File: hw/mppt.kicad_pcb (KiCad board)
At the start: 2 copper layers, 7 parts, among them J1 Conn_01x02, J2 Conn_01x02, Q1 Q_NMOS_DGS, Q2 Q_NMOS_DGS

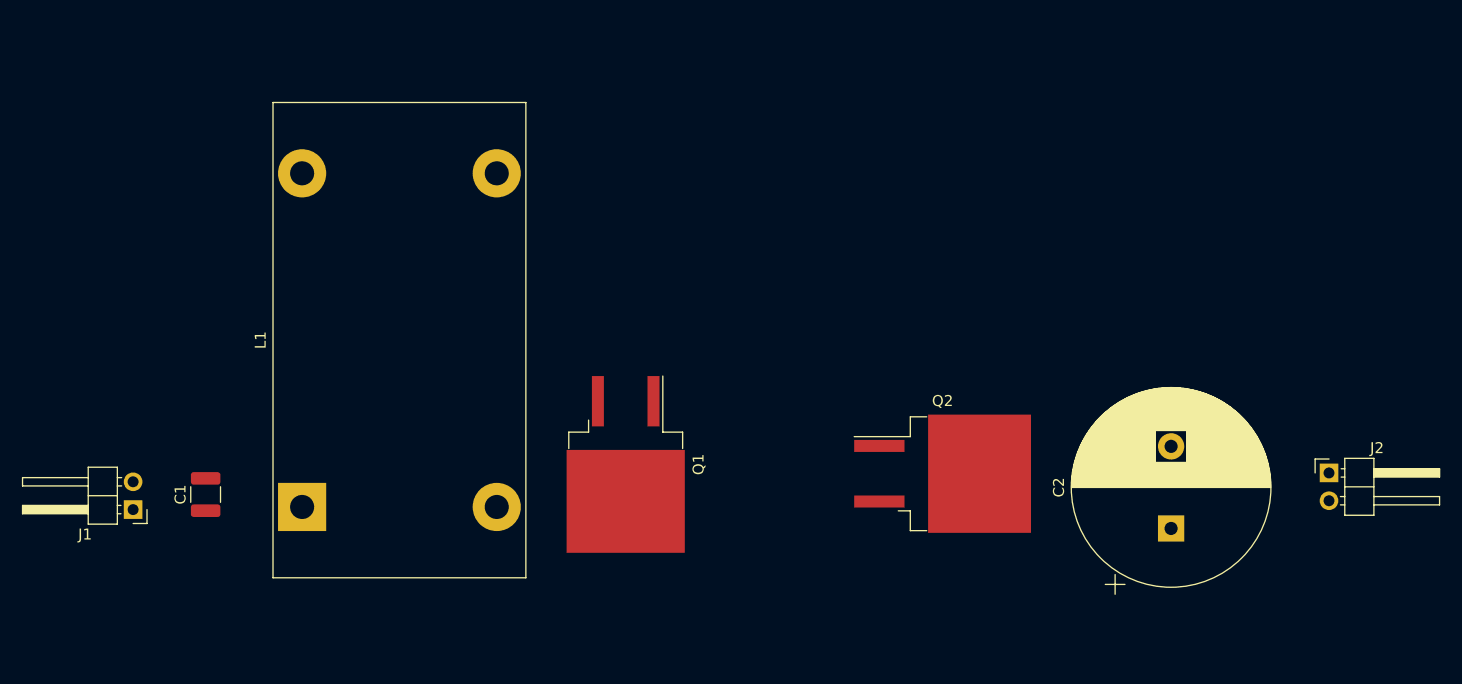
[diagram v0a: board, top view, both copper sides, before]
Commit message: working on documentation, design methmethodology, sizing, layout
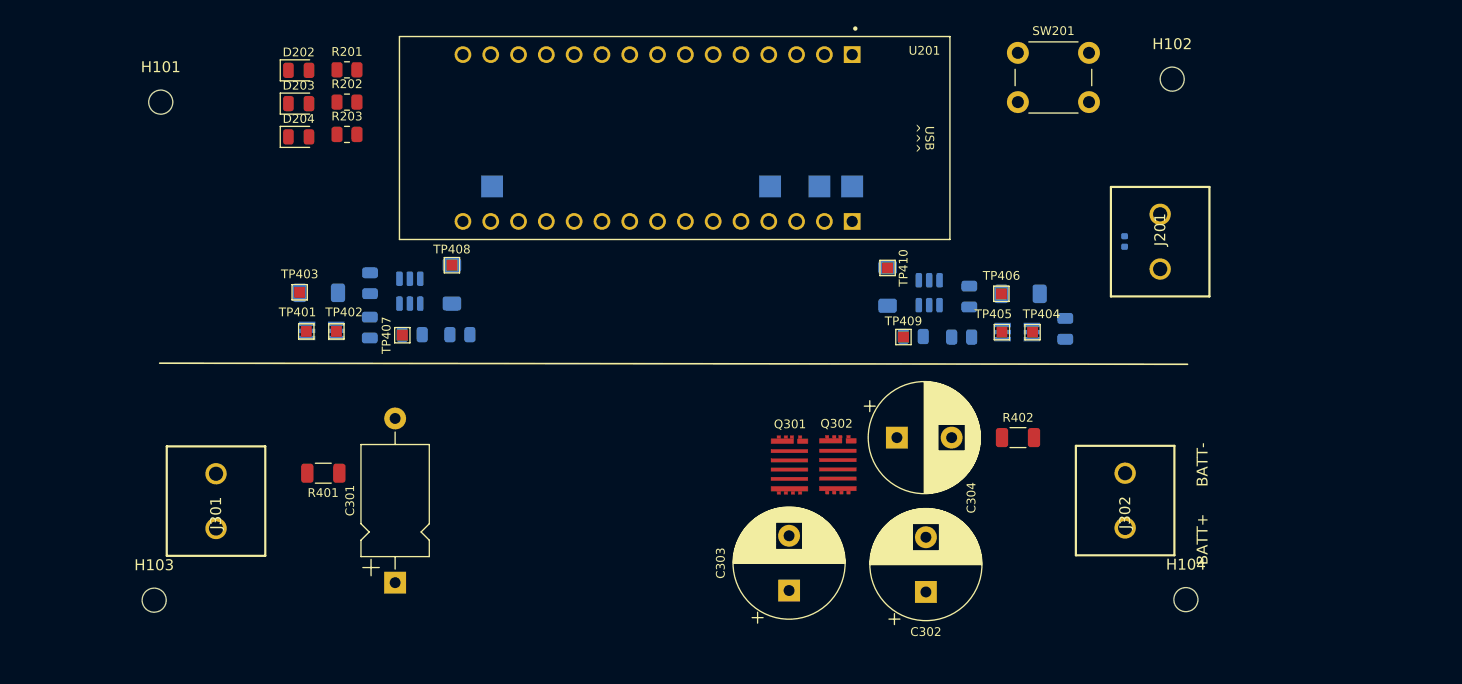
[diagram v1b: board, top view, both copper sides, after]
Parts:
- removed C1: 10uF, Capacitor_SMD:C_1210_3225Metric
- removed C2: 330uF, Capacitor_THT:CP_Radial_D18.0mm_P7.50mm
- removed J1, J2: Conn_01x02, Connector_PinHeader_2.54mm:PinHeader_1x02_P2.54mm_Horizontal
- removed L1: 1529uH, Inductor_THT:L_CommonMode_Toroid_Vertical_L43.2mm_W22.9mm_Px17.78mm_Py30.48mm_Bourns_8100
- removed Q1, Q2: Q_NMOS_DGS, Package_TO_SOT_SMD:TO-263-2
- added C201: 100nF, Capacitor_SMD:C_0402_1005Metric, B.Cu at (183.2, 77.6)
- added C301: 5uF, Capacitor_THT:CP_Axial_L10.0mm_D6.0mm_P15.00mm_Horizontal, F.Cu at (116.5, 108.8)
- added C302: 18uF, Capacitor_THT:CP_Radial_D10.0mm_P5.00mm, F.Cu at (165.0, 109.6)
- added C303: 18uF, Capacitor_THT:CP_Radial_D10.0mm_P5.00mm, F.Cu at (152.5, 109.5)
- added C304: 18uF, Capacitor_THT:CP_Radial_D10.0mm_P5.00mm, F.Cu at (162.3, 95.5)
- added C401: 100nF, Capacitor_SMD:C_0805_2012Metric, B.Cu at (114.2, 85.4)
- added C402: 100nF, Capacitor_SMD:C_0805_2012Metric, B.Cu at (177.7, 85.6)
- added C403: 100nF, Capacitor_SMD:C_0805_2012Metric, B.Cu at (114.2, 81.4)
- added C404: 100nF, Capacitor_SMD:C_0805_2012Metric, B.Cu at (169.0, 82.6)
- added D202: BLUE, LED_SMD:LED_0805_2012Metric, F.Cu at (107.7, 61.9)
- added D203: YELLOW, LED_SMD:LED_0805_2012Metric, F.Cu at (107.7, 65.0)
- added D204: RED, LED_SMD:LED_0805_2012Metric, F.Cu at (107.7, 68.0)
- added D401: 3.3V Zener, Diode_SMD:D_MiniMELF, B.Cu at (109.5, 82.3)
- added D402: 3.3V Zener, Diode_SMD:D_MiniMELF, B.Cu at (173.6, 82.4)
- added D403: 3.3V Zener, Diode_SMD:D_MiniMELF, B.Cu at (121.7, 81.5)
- added D404: 3.3V Zener, Diode_SMD:D_MiniMELF, B.Cu at (161.5, 81.7)
- added H101: Top Left Mounting Hole, MountingHole:MountingHole_2.2mm_M2, F.Cu at (95.1, 64.9)
- added H102: Top Right Mounting Hole, MountingHole:MountingHole_2.2mm_M2, F.Cu at (187.5, 62.8)
- added H103: Bottom Left Mounting Hole, MountingHole:MountingHole_2.2mm_M2, F.Cu at (94.5, 110.3)
- added H104: Bottom Right Mounting Hole, MountingHole:MountingHole_2.2mm_M2, F.Cu at (188.8, 110.3)
- added J201: 1935776, mppt:1935776, F.Cu at (186.4, 75.1)
- added J301: 1935776, mppt:1935776, F.Cu at (100.2, 103.8)
- added J302: 1935776, mppt:1935776, F.Cu at (183.2, 103.8)
- added Q301: Q_NMOS_DGS, mppt:EPC2307, F.Cu at (152.5, 97.8)
- added Q302: Q_NMOS_DGS, mppt:EPC2307, F.Cu at (156.9, 97.8)
- added R201: 330, Resistor_SMD:R_0805_2012Metric, F.Cu at (112.1, 61.9)
- added R202: 330, Resistor_SMD:R_0805_2012Metric, F.Cu at (112.1, 64.9)
- added R203: 330, Resistor_SMD:R_0805_2012Metric, F.Cu at (112.1, 67.8)
- added R401: 2m, Resistor_SMD:R_1206_3216Metric, F.Cu at (110.0, 98.8)
- added R402: 2m, Resistor_SMD:R_1206_3216Metric, F.Cu at (173.4, 95.5)
- added R403: 100k, Resistor_SMD:R_0805_2012Metric, B.Cu at (118.1, 86.1)
- added R404: 3k, Resistor_SMD:R_0805_2012Metric, B.Cu at (122.4, 86.1)
- added R405: 100k, Resistor_SMD:R_0805_2012Metric, B.Cu at (163.8, 86.3)
- added R406: 2k, Resistor_SMD:R_0805_2012Metric, B.Cu at (168.3, 86.3)
- added SW201: SW_Push, Button_Switch_THT:SW_PUSH_6mm, F.Cu at (173.4, 60.4)
- added TP201: 3.3V TP, TestPoint:TestPoint_Pad_2.0x2.0mm, B.Cu at (125.4, 72.5)
- added TP202: 12V TP, TestPoint:TestPoint_Pad_2.0x2.0mm, B.Cu at (158.3, 72.5)
- added TP203: 5V TP, TestPoint:TestPoint_Pad_2.0x2.0mm, B.Cu at (150.8, 72.5)
- added TP204: GND MCU TP, TestPoint:TestPoint_Pad_2.0x2.0mm, B.Cu at (155.3, 72.5)
- added TP401: GND, TestPoint:TestPoint_Pad_1.0x1.0mm, F.Cu at (108.4, 85.8)
- added TP402: -ARR, TestPoint:TestPoint_Pad_1.0x1.0mm, F.Cu at (111.1, 85.8)
- added TP403: Array Current, TestPoint:TestPoint_Pad_1.0x1.0mm, F.Cu at (107.8, 82.2)
- added TP404: -BATT, TestPoint:TestPoint_Pad_1.0x1.0mm, F.Cu at (174.7, 85.9)
- added TP405: GND, TestPoint:TestPoint_Pad_1.0x1.0mm, F.Cu at (171.9, 85.9)
- added TP406: Battery Current, TestPoint:TestPoint_Pad_1.0x1.0mm, F.Cu at (171.9, 82.4)
- added TP407: +ARR, TestPoint:TestPoint_Pad_1.0x1.0mm, F.Cu at (117.2, 86.1)
- added TP408: Array Voltage, TestPoint:TestPoint_Pad_1.0x1.0mm, F.Cu at (121.7, 79.8)
- added TP409: +BATT, TestPoint:TestPoint_Pad_1.0x1.0mm, F.Cu at (162.9, 86.3)
- added TP410: Battery Voltage, TestPoint:TestPoint_Pad_1.0x1.0mm, F.Cu at (161.5, 80.0)
- added U201: MCU_Nucleo_L432KC, mppt:MODULE_NUCLEO-L432KC, F.Cu at (142.1, 68.1)
- added U401: INA210, Package_TO_SOT_SMD:SOT-363_SC-70-6_Handsoldering, B.Cu at (109.8, 85.8)
- added U402: INA210, Package_TO_SOT_SMD:SOT-363_SC-70-6_Handsoldering, B.Cu at (173.3, 85.9)
- added U403: OPA990, Package_TO_SOT_SMD:SOT-23-6, B.Cu at (117.9, 82.1)
- added U404: OPA990, Package_TO_SOT_SMD:SOT-23-6, B.Cu at (165.3, 82.3)
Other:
- copper layers 2 -> 4
- board text added: "BATT+"
- board text added: "BATT-"
- board text added: "Gate Driver"
- board text added: "Inductor"
- board text added: "Sizing for RM8 Core"
- board text added: "USB ^^^"
- board text added: "VIA FENCE"
- board text removed: "Array Measurement Circuitry"
- board text removed: "Battery Measurement Circuitry"
- board text removed: "Controller"
- board text removed: "Oversized inductor region"

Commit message: parts of gate driver
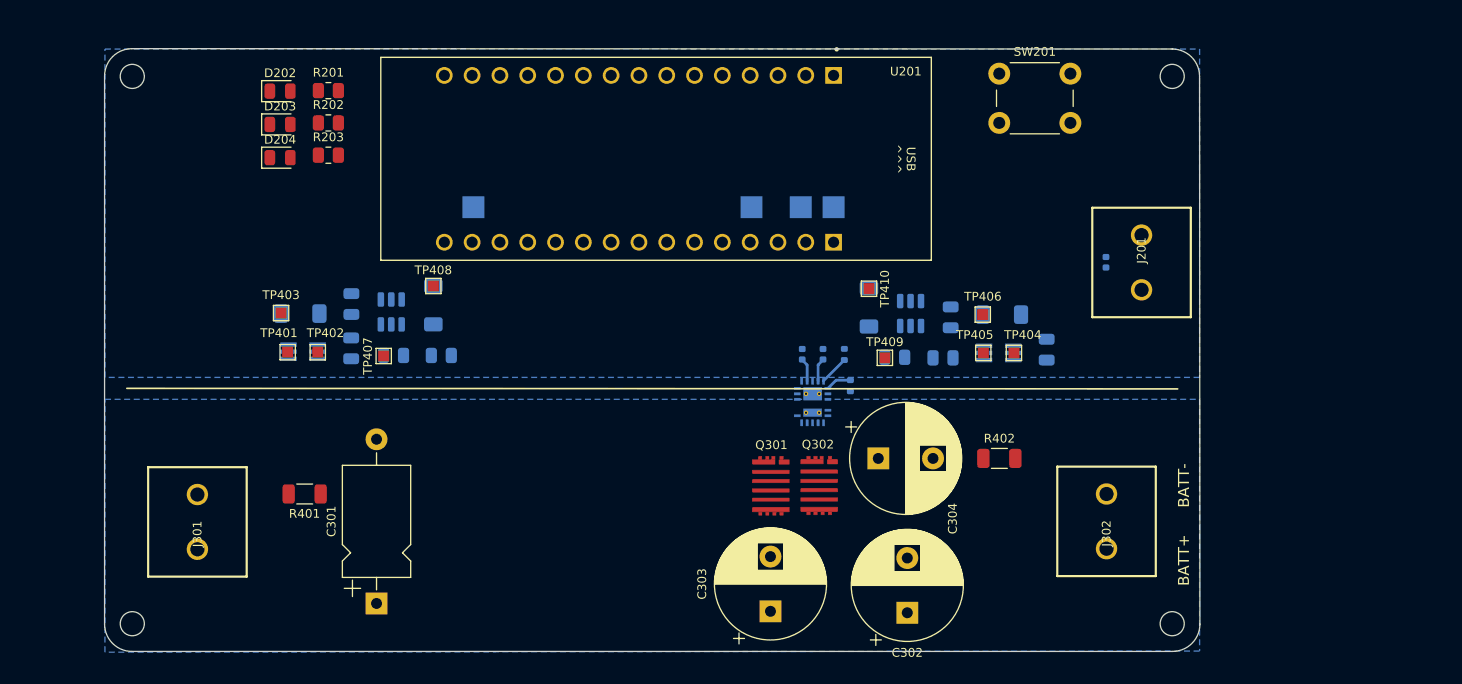
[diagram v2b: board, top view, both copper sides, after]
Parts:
- added C501: 10uF, Capacitor_SMD:C_0402_1005Metric, B.Cu at (155.6, 87.9)
- added C502: 10uF, Capacitor_SMD:C_0402_1005Metric, B.Cu at (153.7, 87.9)
- added R501: 20k, Resistor_SMD:R_0402_1005Metric, B.Cu at (158.1, 90.8)
- added R502: 20k, Resistor_SMD:R_0402_1005Metric, B.Cu at (157.6, 87.9)
- added U501: LMG1210RVRT, mppt:IC_LMG1210RVRT, B.Cu at (154.7, 92.2)
- moved H101 3.51 mm to (92.5, 62.5)
- moved H103 2.94 mm to (92.5, 112.5)
- moved C201 2.55 mm to (181.4, 79.5)
- moved C404 2.55 mm to (167.3, 84.5)
- moved D402 2.55 mm to (171.9, 84.3)
- moved J201 2.55 mm to (184.7, 77.0)
- moved TP404 2.55 mm to (173.0, 87.8)
- moved TP406 2.55 mm to (170.2, 84.3)
- moved U201 2.55 mm to (140.3, 70.0)
- moved SW201 2.55 mm to (171.7, 62.2)
- moved C403 2.55 mm to (112.5, 83.3)
- moved D203 2.55 mm to (106.0, 66.9)
- moved D401 2.55 mm to (107.8, 84.2)
- moved J301 2.55 mm to (98.5, 105.7)
- moved R203 2.55 mm to (110.4, 69.7)
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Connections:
- U201 pad 19: unconnected-(U201-A0-Pad19) -> /controller/PWM_EN
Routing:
- net Net-(U501-DHL): track 0.00 -> 2.72 mm
- net Net-(U501-DLH): track 0.00 -> 2.36 mm
- net +5V: track 0.00 -> 2.19 mm
- net +12V: track 0.00 -> 2.19 mm
- added copper zone on B.Cu, net GND
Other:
- board outline added: 100.1 x 55.1 mm
